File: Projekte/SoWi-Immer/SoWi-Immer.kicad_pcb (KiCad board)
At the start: 2 copper layers, 42 x 12.3 mm, 14 parts, among them P1 CONN_01X02, U1 SPV1040

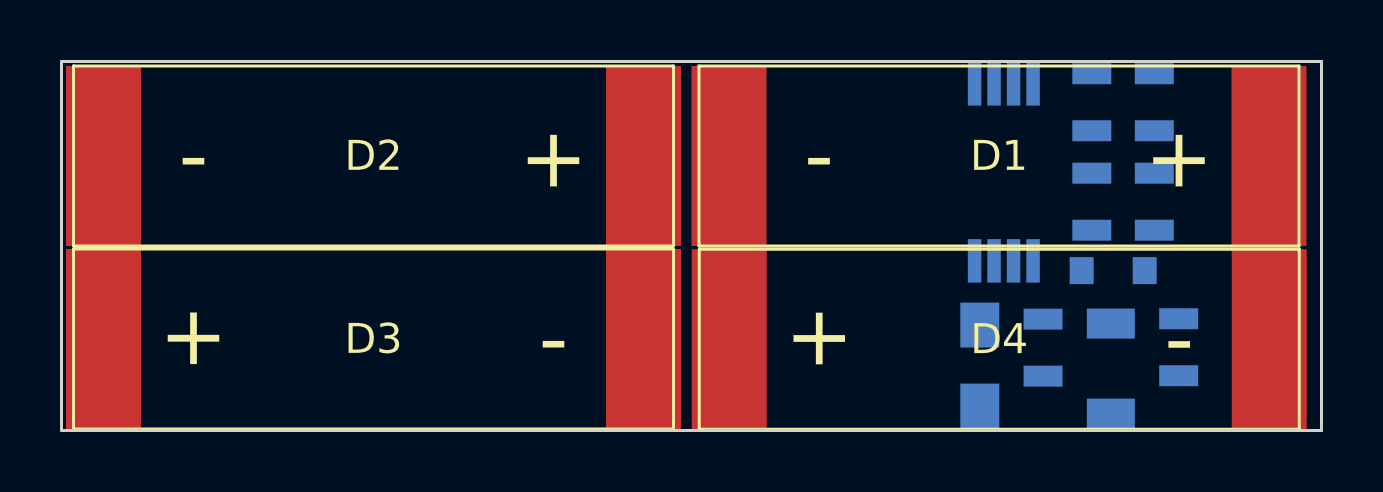
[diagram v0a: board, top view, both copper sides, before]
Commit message: Diverse Dateien hinzugefügt
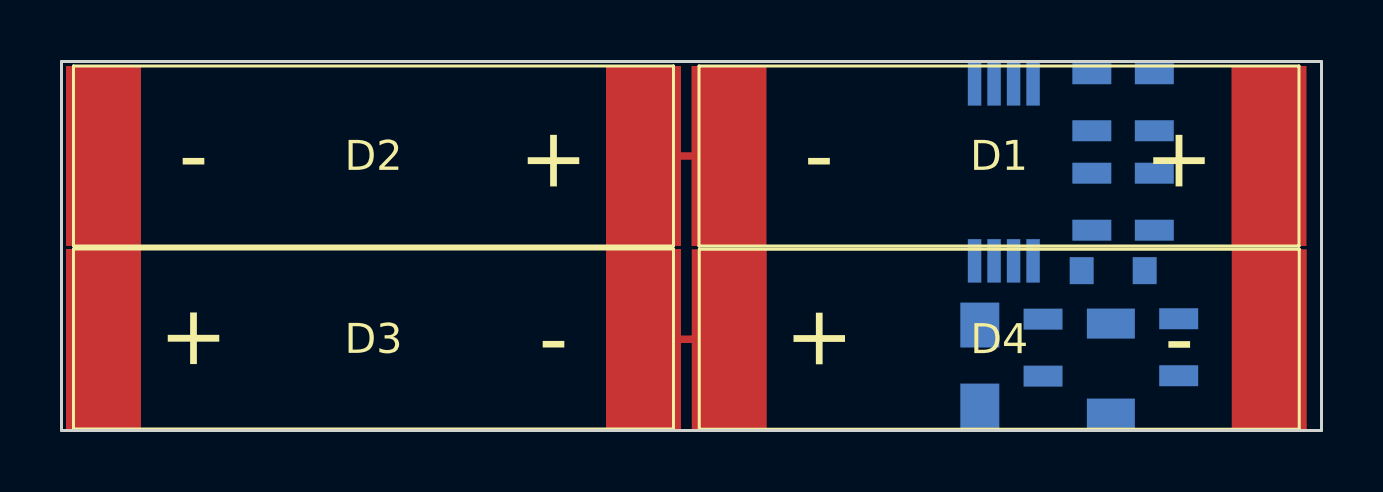
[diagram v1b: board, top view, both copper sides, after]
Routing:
- net Net-(D2-Pad2): track 0.00 -> 6.10 mm
- net Net-(D3-Pad2): track 0.00 -> 2.86 mm
- net Net-(D1-Pad2): track 0.00 -> 2.85 mm
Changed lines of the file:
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@@
   (general
     (links 23)
-    (no_connects 23)
-    (area 139.949999 79.949999 182.050001 92.350001)
+    (no_connects 20)
+    (area 139.949999 78.158599 182.050001 94.558033)
     (thickness 1.6)
     (drawings 4)
-    (tracks 0)
+    (tracks 4)
     (zones 0)
     (modules 14)
@@
   (gr_line (start 182 80) (end 182 92.3) (angle 90) (layer Edge.Cuts) (width 0.1))
   (gr_line (start 140 80) (end 140 92.3) (angle 90) (layer Edge.Cuts) (width 0.1))
+  (segment (start 159.4 83.15) (end 162.25 83.15) (width 0.25) (layer F.Cu) (net 4) (status C00000))
+  (segment (start 141.4 83.15) (end 141.4 89.25) (width 0.25) (layer F.Cu) (net 5) (status C00000))
+  (segment (start 162.2581 89.258) (end 159.408 89.258) (width 0.25) (layer F.Cu) (net 6) (status C00000))
+  (segment (start 159.408 89.258) (end 159.4 89.25) (width 0.25) (layer F.Cu) (net 6) (status C00000))
 )
